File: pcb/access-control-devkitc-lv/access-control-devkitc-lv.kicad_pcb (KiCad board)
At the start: 2 copper layers, 57.6 x 65.5 mm, 32 parts, among them J1 CON_I2C, U1 ESP32-DevKitC

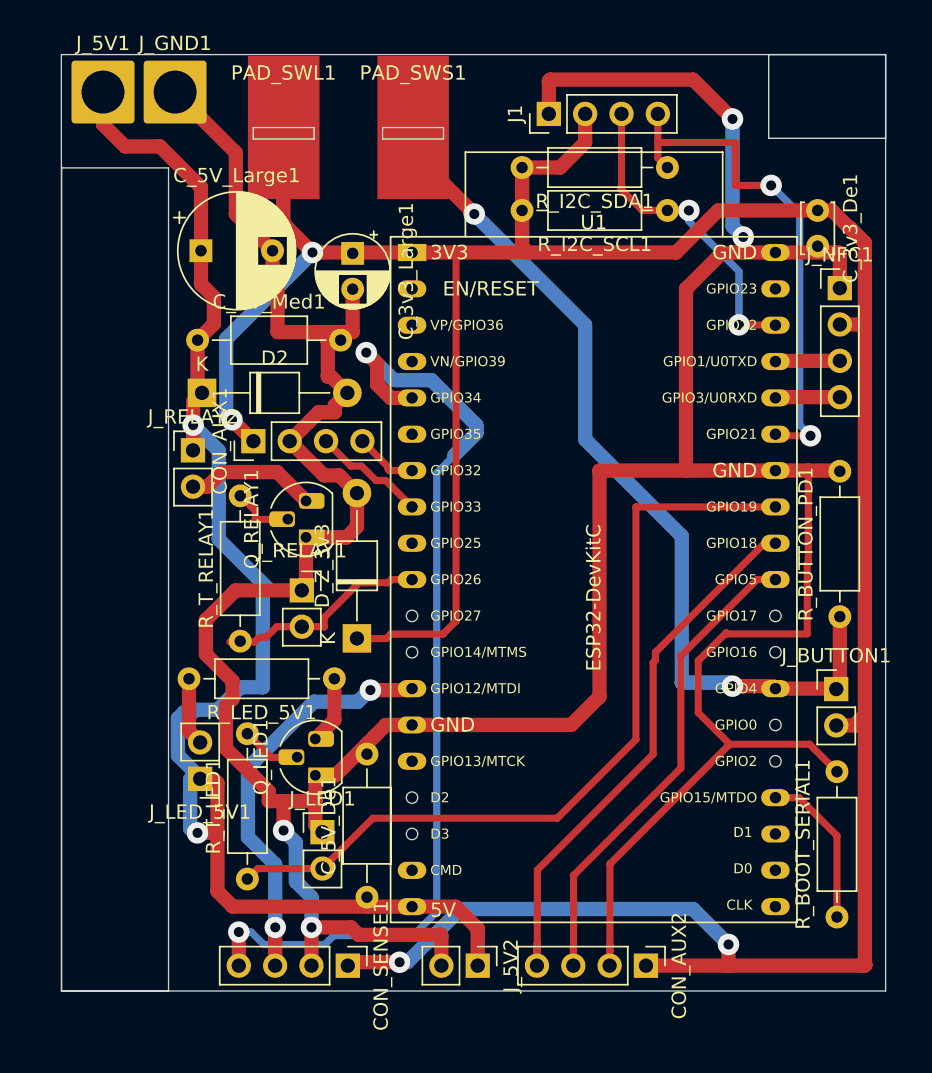
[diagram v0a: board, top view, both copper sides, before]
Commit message: Update with values
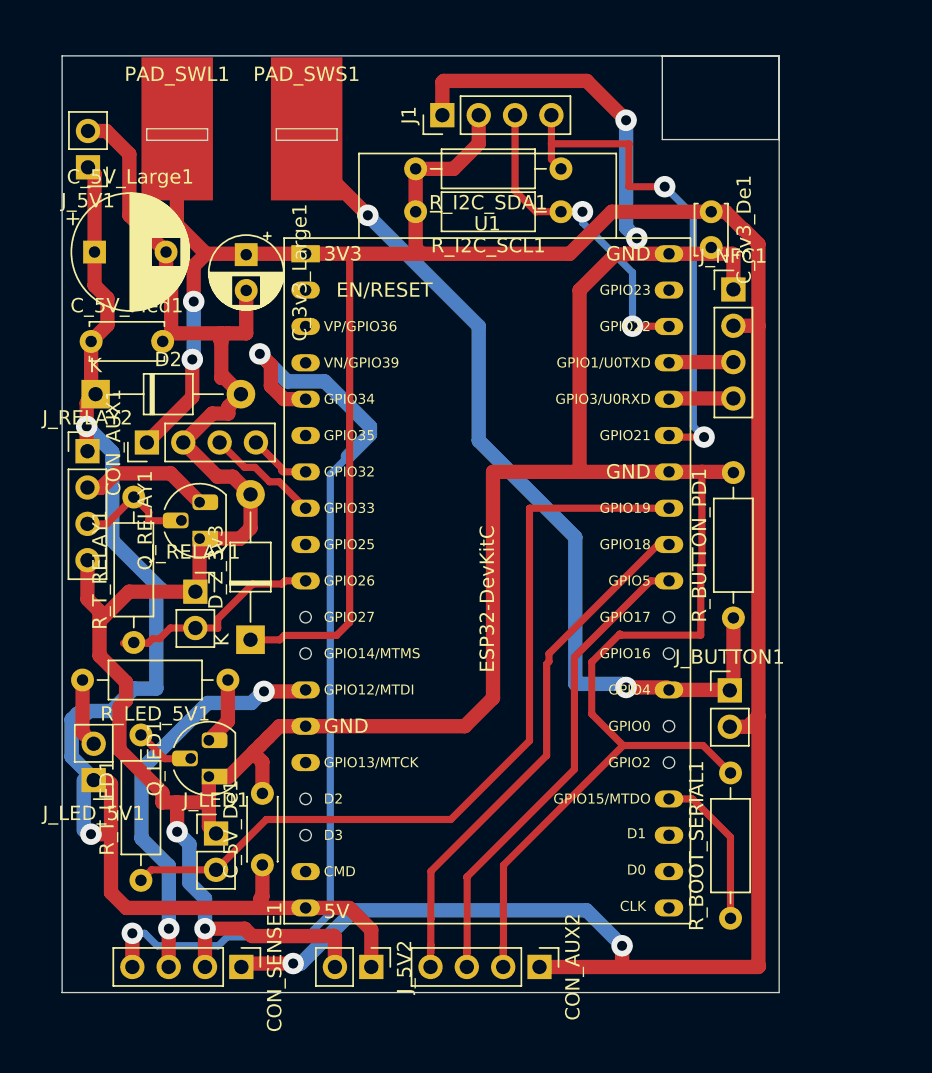
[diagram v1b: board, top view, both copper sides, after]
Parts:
- removed J_GND1: Conn_01x01_Socket, Connector_Wire:SolderWire-2.5sqmm_1x01_D2.4mm_OD4.4mm
- C_5V_De1: footprint Capacitor_THT:C_Axial_L5.1mm_D3.1mm_P10.00mm_Horizontal -> Capacitor_THT:C_Disc_D4.3mm_W1.9mm_P5.00mm
- C_5V_Med1: footprint Capacitor_THT:C_Axial_L5.1mm_D3.1mm_P10.00mm_Horizontal -> Capacitor_THT:C_Disc_D5.0mm_W2.5mm_P5.00mm
- J_5V1: value Conn_01x01_Socket -> Conn_01x02_Socket; footprint Connector_Wire:SolderWire-2.5sqmm_1x01_D2.4mm_OD4.4mm -> Connector_PinHeader_2.54mm:PinHeader_1x02_P2.54mm_Vertical
- J_RELAY2: footprint Connector_PinHeader_2.54mm:PinHeader_1x02_P2.54mm_Vertical -> Connector_PinHeader_2.54mm:PinHeader_1x04_P2.54mm_Vertical
- moved C_5V_De1 7.65 mm to (14.1, 56.6)
- moved J1 7.44 mm to (26.6, 4.22)
- moved J_5V2 7.44 mm to (21.7, 63.8)
- moved PAD_SWS1 7.44 mm to (17.1, 5.18)
- moved Q_RELAY1 7.44 mm to (9.66, 33.8)
- moved U1 7.44 mm to (17.1, 13.9)
- moved CON_AUX1 7.44 mm to (5.98, 27.1)
- moved CON_SENSE1 7.44 mm to (12.6, 63.8)
- moved C_3v3_Large1 7.44 mm to (12.9, 14.0)
- moved C_5V_Large1 7.44 mm to (2.32, 13.8)
- moved C_5V_Med1 7.44 mm to (2.08, 20.0)
- moved D2 7.44 mm to (2.39, 23.7)
- moved D_Z_3v3 7.44 mm to (13.2, 40.9)
- moved J_LED1 7.44 mm to (10.8, 54.4)
- moved J_LED_5V1 7.44 mm to (2.26, 50.7)
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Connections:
- Q_RELAY1 pad 2: Net-(Q_RELAY1-B) -> Net-(J_RELAY2-Pin_3)
- R_T_RELAY1 pad 2: Net-(Q_RELAY1-B) -> Net-(J_RELAY2-Pin_3)
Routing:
- net Net-(J_RELAY2-Pin_3): track 0.00 -> 7.84 mm
- net +5V: track 98.3 -> 91.4 mm
- net GND: track 271.4 -> 277.5 mm
- net Net-(Q_RELAY1-B): track 3.83 -> 0.00 mm
- net +3V3: track 214.1 -> 212.5 mm
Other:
- board size 57.6 x 65.5 mm -> 50.1 x 65.5 mm
